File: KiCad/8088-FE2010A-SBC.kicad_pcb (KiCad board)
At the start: 2 copper layers, 127 x 111.8 mm, 61 parts, among them P1 KEYBOARD, P2 SPEAKER, P3 RESET, Q1 PN2222A, SW1 RESET, SW2 CONFIG, U1 8088, U10 74ALS245, U11 74ALS245, U12 74ALS244, U13 74ALS244, U14 74ALS04, U15 PIC12F629, U2 8087, U3 FE2010A, U4 28C256, U5 AS6C4008, U6 AS6C1008, U7 74LS573, U8 74LS573, X1 28.63636MHz

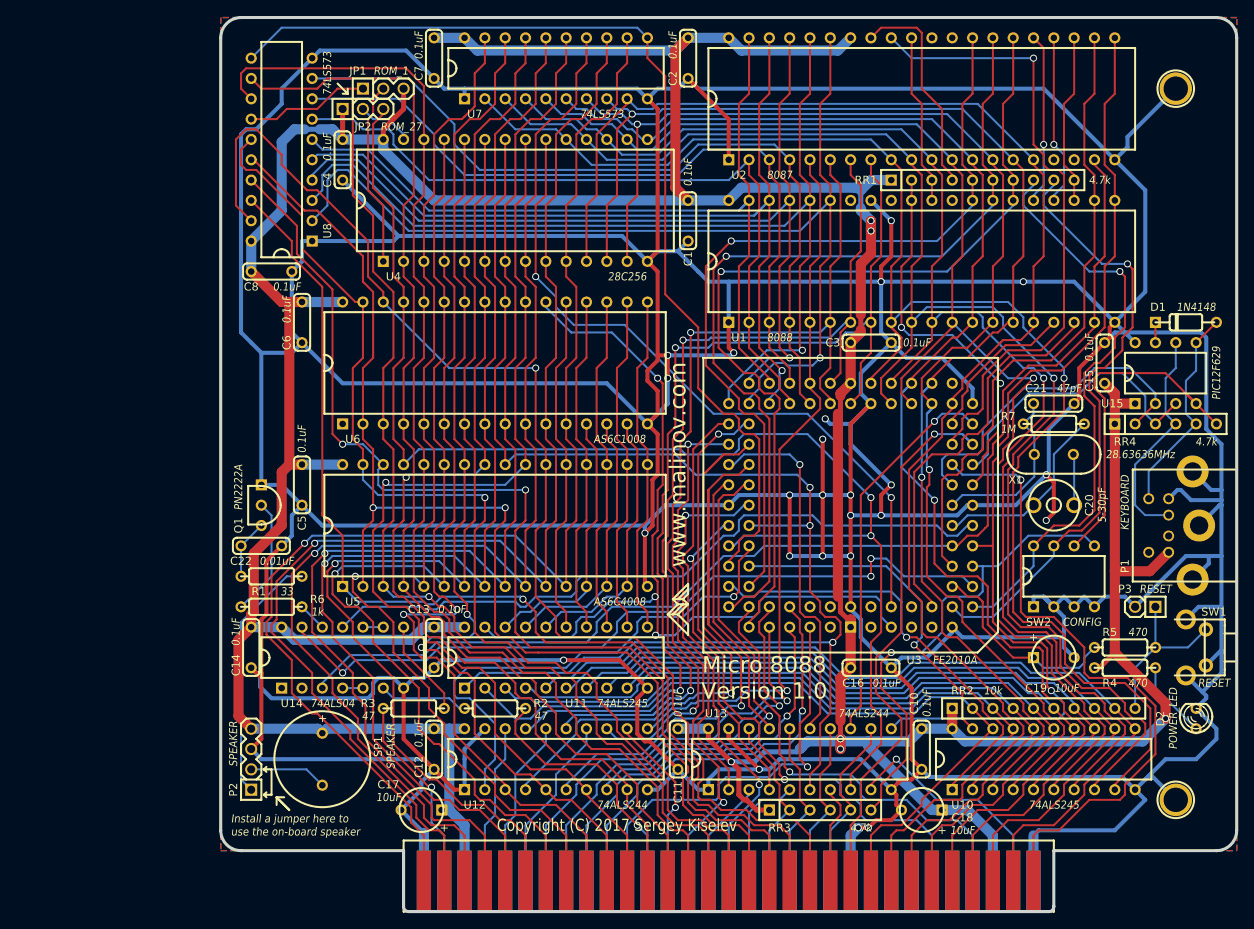
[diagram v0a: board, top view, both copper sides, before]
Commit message: Add 1.1 files
Signed-off-by: Sergey Kiselev <sergey.kiselev@intel.com>
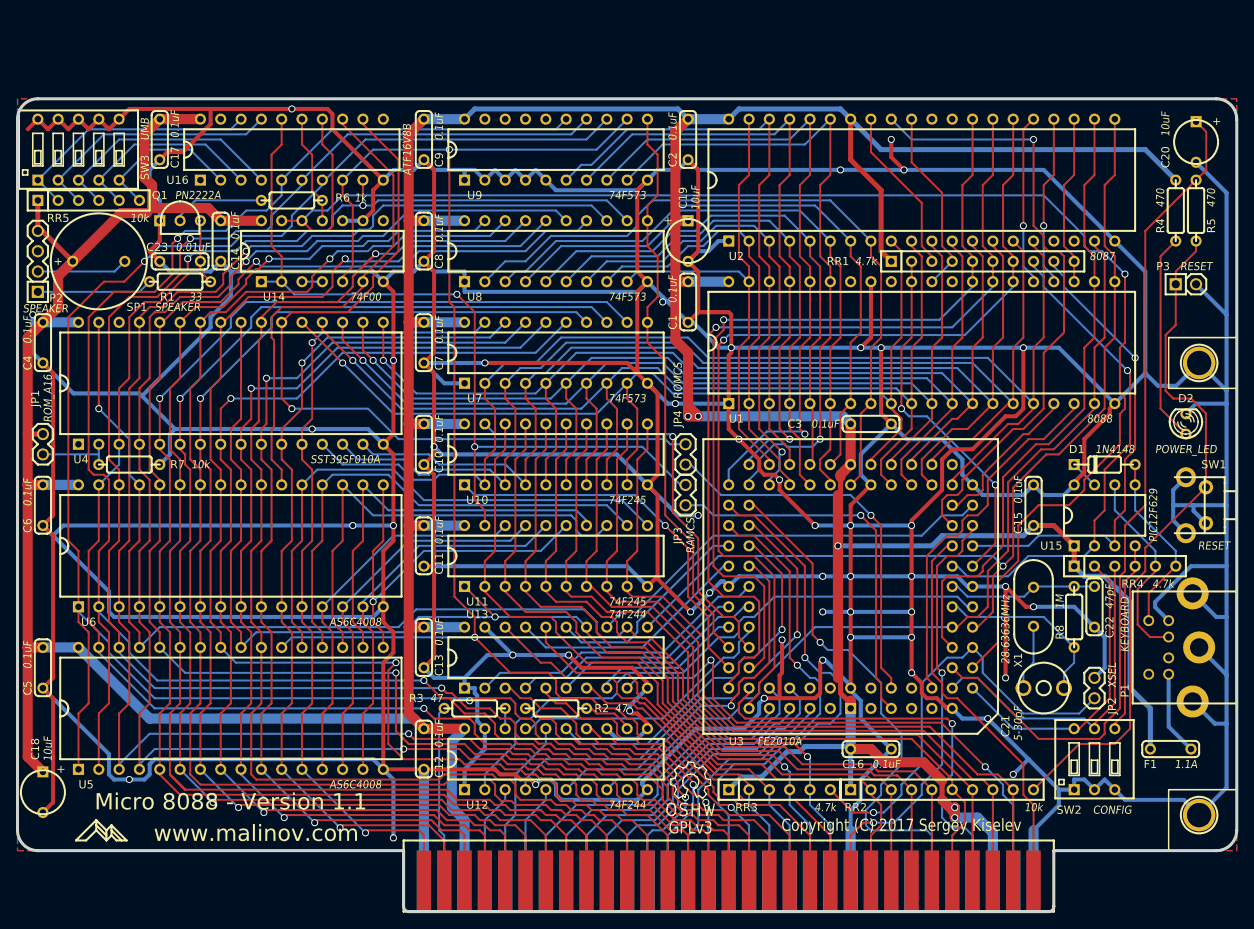
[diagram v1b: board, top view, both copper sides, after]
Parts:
- added C17: 0.1uF, my_components:Cap_Cer_508, F.Cu at (76.2, 53.3)
- added C9: 0.1uF, my_components:Cap_Cer_508, F.Cu at (109.2, 53.3)
- added F1: 1.1A, my_components:Cap_Cer_508, F.Cu at (202.6, 129.5)
- added GPLv3: Symbol_OSHW-Logo_SilkScreen, Symbols:Symbol_OSHW-Logo_SilkScreen, F.Cu at (142.6, 133.7)
- added JP3: RAMCS, my_components:Conn_Pin_Header_2x1_2.54mm_NoKey, F.Cu at (141.9, 97.8)
- added JP4: ROMCS, my_components:Conn_Pin_Header_2x1_2.54mm_NoKey, F.Cu at (141.9, 92.7)
- added R8: 1M, my_components:Res_762, F.Cu at (190.5, 113.0)
- added RR5: 10k, my_components:Conn_SIL6, F.Cu at (67.3, 61.0)
- added SW3: UMB, my_components:Switch_DIP_5_Positions, F.Cu at (66.0, 54.6)
- added U16: ATF16V8B, my_components:IC_DIP20_300, F.Cu at (92.7, 54.6)
- added U9: 74F573, my_components:IC_DIP20_300, F.Cu at (125.7, 54.6)
- JP1: value ROM_1 -> ROM_A16; footprint my_components:Conn_Pin_Header_3x1_2.54mm -> my_components:Conn_Pin_Header_2x1_2.54mm_NoKey
- JP2: value ROM_27 -> XSEL; footprint my_components:Conn_Pin_Header_3x1_2.54mm -> my_components:Conn_Pin_Header_2x1_2.54mm_NoKey
- R7: value 1M -> 10k
- SW2: footprint my_components:IC_DIP8_300 -> my_components:Switch_DIP_3_Positions
- U10, U11: value 74ALS245 -> 74F245
- U12, U13: value 74ALS244 -> 74F244
- U14: value 74ALS04 -> 74F00
- U4: value 28C256 -> SST39SF010A; footprint my_components:IC_DIP28_600 -> my_components:IC_DIP32_600
- U6: value AS6C1008 -> AS6C4008
- U7, U8: value 74LS573 -> 74F573
- moved JP2 116.6 mm to (193.0, 121.9), turned to 270 degrees
- moved R7 115.7 mm to (72.4, 94.0), turned to 180 degrees
- moved C19 76.9 mm to (142.2, 66.0), turned to 270 degrees
- moved C10 73.0 mm to (109.2, 91.4)
- moved U10 71.9 mm to (125.7, 92.7)
- moved SP1 68.2 mm to (68.6, 68.6), turned to 0 degrees
- moved P2 67.7 mm to (61.0, 68.6)
- moved C20 66.9 mm to (205.7, 53.7), turned to 270 degrees
- moved JP1 61.5 mm to (61.6, 91.4), turned to 90 degrees
- moved R4 57.5 mm to (203.2, 62.2), turned to 270 degrees
- moved R5 55.3 mm to (205.7, 62.2), turned to 270 degrees
- moved C14 50.9 mm to (83.8, 66.0)
- moved R6 50.9 mm to (92.7, 61.0)
- moved U14 50.9 mm to (96.5, 67.3)
- moved C18 47.4 mm to (61.6, 134.9), turned to 270 degrees
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- renumbered C17 to C18, C18 to C19, C19 to C20, C20 to C21, C21 to C22, C22 to C23
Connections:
- C21 pad 2: Net-(C20-Pad2) -> Net-(C21-Pad2)
- C22 pad 1: Net-(C21-Pad1) (its old number) -> Net-(C22-Pad1)
- JP1 pad 1: /A14 -> /ROM_A16
- JP1 pad 2: /ROM_1 -> VCC
- JP2 pad 1: VCC -> GND
- JP2 pad 2: /ROM_27 -> /XSEL
- P1 pad 4: VCC -> /KBD_VCC
- P2 pad 3: GND -> Net-(P2-Pad3)
- R6 pad 2: Net-(R6-Pad2) -> /~SPKR
- R7 pad 1: Net-(C21-Pad1) (its old number) -> GND
- R7 pad 2: Net-(C20-Pad2) -> /ROM_A16
- RR1 pad 3: /~RQ/GT1 -> /~RQ/GT2
- RR1 pad 4: /~RQ/GT2 -> /~RQ/GT1
- RR1 pad 8: /~VID0 -> /KBCLK
- RR1 pad 9: /~VID1 -> /KBDATA
- RR4 pad 2: /KBCLK -> /~VID0
- RR4 pad 3: /KBDATA -> /~VID1
- RR4 pad 4: /AT_KBDATA -> /E0_PASS
- RR4 pad 5: /AT_KBCLK -> /AT_KBDATA
- RR4 pad 6: /E0_PASS -> /AT_KBCLK
- SW2 pad 4: GND -> /E0_PASS
- SW2 pad 5: /XSEL -> /~VID1
- SW2 pad 6: /E0_PASS -> /~VID0
- U11 pad 1: /~XMEMR -> /~MEMR
- U11 pad 11: /MD3 -> /MD7
- U11 pad 12: /MD4 -> /MD6
- U11 pad 14: /MD6 -> /MD4
- U11 pad 15: /MD7 -> /MD3
- U11 pad 19: /~RAMCS -> /~RAMENA
- U11 pad 5: /D7 -> /D3
- U11 pad 6: /D6 -> /D4
- U11 pad 8: /D4 -> /D6
- U11 pad 9: /D3 -> /D7
- U12 pad 11: /AA11 -> GND
- U12 pad 12: /~DACK0 -> Net-(R2-Pad2)
- U12 pad 13: /AA10 -> GND
- U12 pad 14: /~DACK2 -> /~DACK0
- U12 pad 15: /AA9 -> /~XDACK2
- U12 pad 17: /AA8 -> /XALE
- U12 pad 18: /ALE -> Net-(R3-Pad2)
- U12 pad 2: /XALE -> /OSC
- U12 pad 3: /A8 -> /ALE
- U12 pad 5: /A9 -> /~DACK2
- U12 pad 6: /~XDACK2 -> /~XDACK0
- U12 pad 7: /A10 -> Net-(U12-Pad7)
- U12 pad 8: /~XDACK0 -> /CLK88
- U12 pad 9: /A11 -> Net-(U12-Pad9)
- U14 pad 1: Net-(U14-Pad1) -> /~RAMENA
- U14 pad 10: Net-(U14-Pad10) -> GND
- U14 pad 11: /OSC -> /~SPKR
- U14 pad 12: Net-(R6-Pad2) -> /SPKR
- U14 pad 2: Net-(U14-Pad2) -> /~RAMENA
- U14 pad 3: /CLK88 -> Net-(U14-Pad3)
- U14 pad 4: Net-(U14-Pad4) -> Net-(U14-Pad3)
- U14 pad 5: Net-(U14-Pad4) -> /A19
- U14 pad 6: Net-(R2-Pad2) -> /~RAMCS2
- U14 pad 8: Net-(R3-Pad2) -> Net-(U14-Pad8)
- U14 pad 9: Net-(U14-Pad10) -> GND
- U3 pad 21: Net-(C20-Pad2) -> Net-(C21-Pad2)
- U3 pad 23: Net-(C21-Pad1) (its old number) -> Net-(C22-Pad1)
- U3 pad 6: /~ROMCS -> /~EPSL
- U4 pad 1: /ROM_1 -> (no net)
- U4 pad 10: /A0 -> /A2
- U4 pad 11: /AD0 -> /A1
- U4 pad 12: /AD1 -> /A0
- U4 pad 13: /AD2 -> /AD0
- U4 pad 14: GND -> /AD1
- U4 pad 15: /AD3 -> /AD2
- U4 pad 16: /AD4 -> GND
- U4 pad 17: /AD5 -> /AD3
- U4 pad 18: /AD6 -> /AD4
- U4 pad 19: /AD7 -> /AD5
- U4 pad 2: /A12 -> /ROM_A16
- U4 pad 20: /~ROMCS -> /AD6
- U4 pad 21: /A10 -> /AD7
- U4 pad 22: /~XMEMR -> /~ROMCS
- U4 pad 23: /A11 -> /A10
- U4 pad 24: /A9 -> /~MEMR
- U4 pad 25: /A8 -> /A11
- U4 pad 26: /A13 -> /A9
- U4 pad 27: /ROM_27 -> /A8
- U4 pad 28: VCC -> /A13
- U4 pad 3: /A7 -> /A15
- U4 pad 4: /A6 -> /A12
- U4 pad 5: /A5 -> /A7
- U4 pad 6: /A4 -> /A6
- U4 pad 7: /A3 -> /A5
- U4 pad 8: /A2 -> /A4
- U4 pad 9: /A1 -> /A3
- U5 pad 24: /~XMEMR -> /~MEMR
- U5 pad 29: /~XMEMW -> /~MEMW
- U6 pad 1: Net-(U6-Pad1) -> /A18
- U6 pad 22: /~RAMCS -> /~RAMCS2
- U6 pad 24: /~XMEMR -> /~MEMR
- U6 pad 29: /~XMEMW -> /~MEMW
- U6 pad 30: /A19 -> /A17
- U7 pad 12: /A0 -> /A7
- U7 pad 13: /A1 -> /A6
- U7 pad 14: /A2 -> /A5
- U7 pad 15: /A3 -> /A4
- U7 pad 16: /A4 -> /A3
- U7 pad 17: /A5 -> /A2
- U7 pad 18: /A6 -> /A1
- U7 pad 19: /A7 -> /A0
- U7 pad 2: /AD7 -> /AD0
- U7 pad 3: /AD6 -> /AD1
- U7 pad 4: /AD5 -> /AD2
- U7 pad 5: /AD4 -> /AD3
- U7 pad 6: /AD3 -> /AD4
- U7 pad 7: /AD2 -> /AD5
- U7 pad 8: /AD1 -> /AD6
- U7 pad 9: /AD0 -> /AD7
- U8 pad 12: /A12 -> /A15
- U8 pad 13: /A13 -> /A14
- U8 pad 14: /A14 -> /A13
- U8 pad 15: /A15 -> /A12
- U8 pad 16: /A16 -> /A11
- U8 pad 17: /A17 -> /A10
- U8 pad 18: /A18 -> /A9
- U8 pad 19: /A19 -> /A8
- U8 pad 2: /AA19 -> /AA8
- U8 pad 3: /AA18 -> /AA9
- U8 pad 4: /AA17 -> /AA10
- U8 pad 5: /AA16 -> /AA11
- U8 pad 6: /AA15 -> /AA12
- U8 pad 7: /AA14 -> /AA13
- U8 pad 8: /AA13 -> /AA14
- U8 pad 9: /AA12 -> /AA15
- X1 pad 2: Net-(C21-Pad1) (its old number) -> Net-(C22-Pad1)
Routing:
- net GND: track 1252.4 -> 1678.2 mm, vias 24 -> 48
- net /~XMEMR: track 180.8 -> 27.1 mm, vias 3 -> 0
- net /~XMEMW: track 170.1 -> 18.8 mm, vias 2 -> 0
- net /~MEMW: track 22.2 -> 157.7 mm, vias 0 -> 2
- net /~MEMR: track 21.2 -> 143.2 mm, vias 0 -> 2
- net /A18: track 137.8 -> 246.8 mm, vias 1 -> 2
- net /~RAMENA: track 0.00 -> 105.8 mm, vias 0 -> 2
- net /SPKR: track 97.9 -> 189.9 mm, vias 3 -> 1
- net /A16: track 151.2 -> 235.3 mm
- net Net-(C20-Pad1): track 25.3 -> 105.3 mm
- net /A15: track 137.3 -> 215.6 mm, vias 1 -> 3
- net /A17: track 139.3 -> 214.7 mm
- net /A14: track 146.5 -> 212.7 mm, vias 1 -> 2
- net /~RAMCS: track 113.5 -> 48.1 mm, vias 3 -> 1
- net /~RESIN: track 21.0 -> 85.1 mm
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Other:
- board size 127 x 111.8 mm -> 152.4 x 101.6 mm
- board text added: "JP1 - Flash ROM Mapping to 0xF0000-0xFFFFF: Open: Map lower 64 KiB of Flash ROM (default) Closed: Map upper 64 KiB of Flash ROM JP2 - Crystal (X1) Frequency Select: Open: 14.31818 MHz (default) Closed: 28.63636 MHz"
- board text added: "JP3, JP4 - RAM and ROM Chip Select Generation: Open: Use SPLD (U16) Closed: Use FE2010 (U3)"
- board text added: "Micro 8088 - Version 1.1"
- board text added: "SW2.1, SW2.2 - Video mode select: SW2.1 = OFF, SW2.2 = OFF: MDA or Hercules SW2.1 = ON, SW2.2 = OFF: 80x25 CGA SW2.1 = OFF, SW2.2 = ON: 40x25 CGA SW2.1 = ON, SW2.2 = ON: None, EGA or VGA"
- board text added: "SW2.3 - Keyboard 0xE0 scan code pass through: SW2.3 = OFF: Disable; SW1.3 = ON: Enable"
- board text added: "SW3 - UMB Configuration: SW3.1 = ON: Enable 0xC0000-0xC7FFF SW3.2 = ON: Enable 0xC8000-0xCFFFF SW3.3 = ON: Enable 0xD0000-0xD7FFF SW3.4 = ON: Enable 0xD8000-0xDFFFF SW3.5 = ON: Enable 0xE0000-0xEFFFF"
- board text removed: "27C128"
- board text removed: "27C256"
- board text removed: "28C256"
- board text removed: "29C256"
- board text removed: "Install a jumper here to use the on-board speaker"
- board text removed: "JP1"
- board text removed: "JP2"
- board text removed: "Micro 8088 Version 1.0"
- board text removed: "ROM Configuration"
- board text removed: "SW1.1, SW1.2 - Video mode select: SW1.1 = OFF, SW1.2 = OFF: MDA or Hercules SW1.1 = ON, SW1.2 = OFF: 80x25 CGA SW1.1 = OFF, SW1.2 = ON: 40x25 CGA SW1.1 = ON, SW1.2 = ON: None, EGA or VGA"
- board text removed: "SW1.3 - Keyboard 0xE0 scan code pass through: SW1.3 = OFF: Disable; SW1.3 = ON: Enable SW1.4 - Crystal select: SW1.4 = OFF: 14.31818 MHz; SW1.4 = ON: 28.63636 MHz"
